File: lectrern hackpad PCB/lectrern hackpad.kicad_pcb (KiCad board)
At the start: 2 copper layers, 93.8 x 74 mm, 18 parts, among them J1 oled connectors, SW1 SW_Push, SW2 SW_Push, SW3 SW_Push, SW4 SW_Push, SW5 SW_Push, SW6 SW_Push, U1 MOUDLE-SEEEDUINO-XIAO

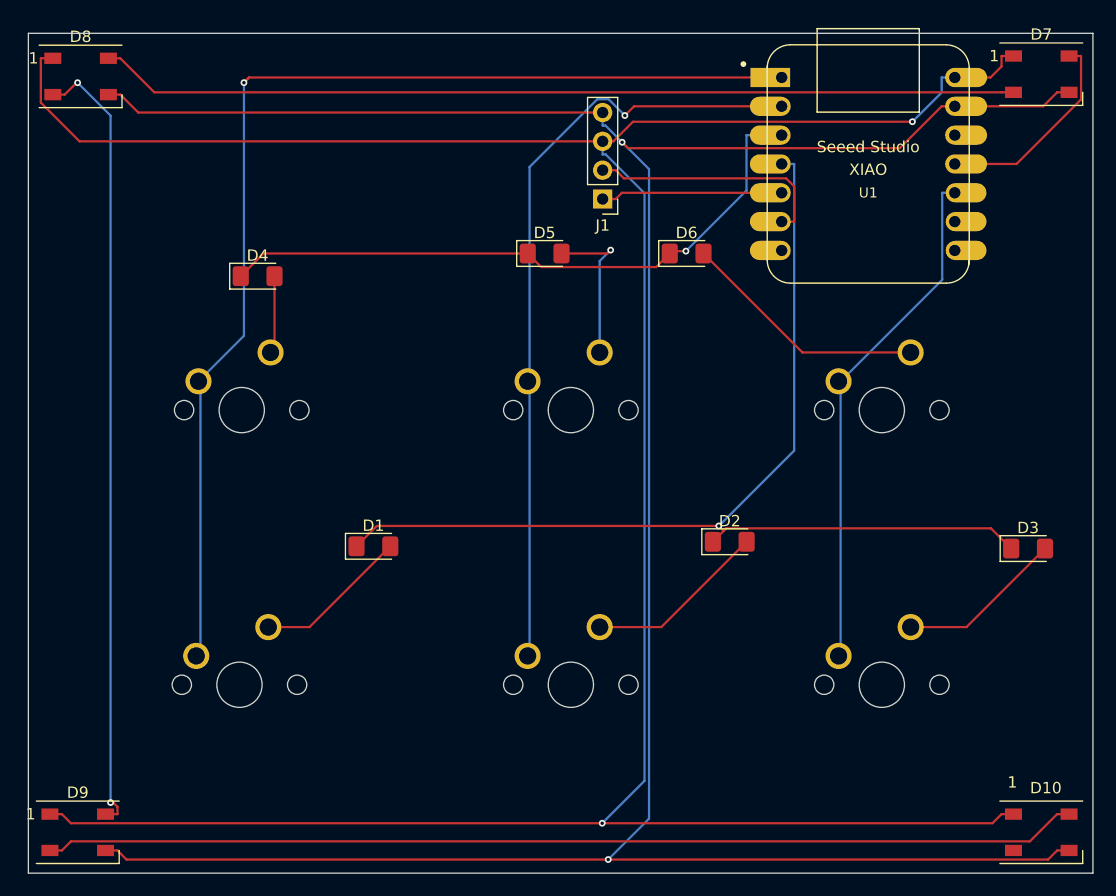
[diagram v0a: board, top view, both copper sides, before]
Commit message: finish all the code firmware
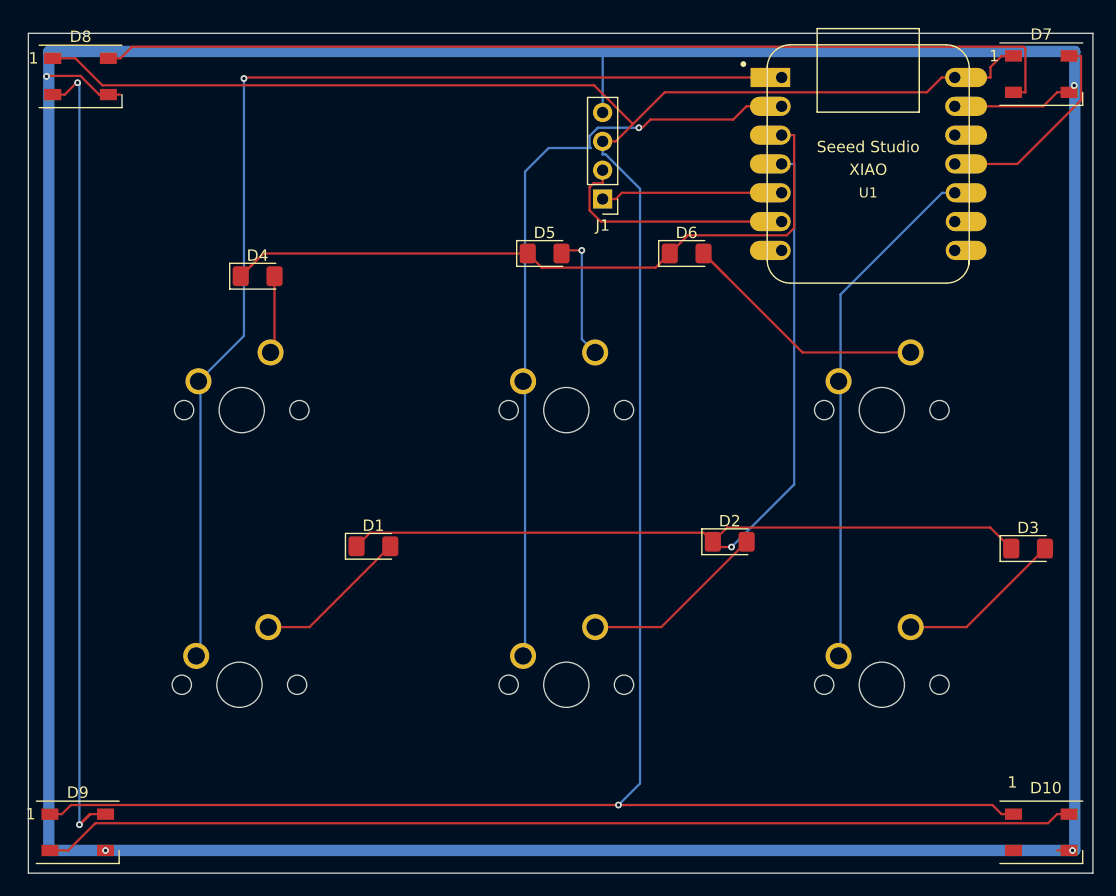
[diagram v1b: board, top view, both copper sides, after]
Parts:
- moved SW3 0.40 mm to (130.0, 68.4)
- moved SW4 0.40 mm to (130.0, 92.6)
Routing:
- net GND: track 240.6 -> 25.3 mm, vias 2 -> 4
- net Row1: track 56.7 -> 63.1 mm, vias 1 -> 0
- net VCC: track 245.4 -> 239.7 mm, vias 2 -> 1
- net Net-(D7-DOUT): track 81.0 -> 86.2 mm
- net Net-(D8-DOUT): track 69.7 -> 73.4 mm
- net Net-(D6-A): track 21.9 -> 24.7 mm
- net Net-(D5-A): track 13.9 -> 11.4 mm
- net Col1: track 102.6 -> 100.2 mm
- net Row2: track 96.5 -> 98.8 mm
- net Col3: track 45.9 -> 46.5 mm
